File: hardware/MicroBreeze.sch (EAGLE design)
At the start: 43 parts, among them IC1 OPA2251UA, IC3 LM2941TO220-V, IC4 LM2941TO220-V, IC5 ATMEGA328P, J1 COMPUTER-PERIPHERAL-POWERVERT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, Y1 16MHZ

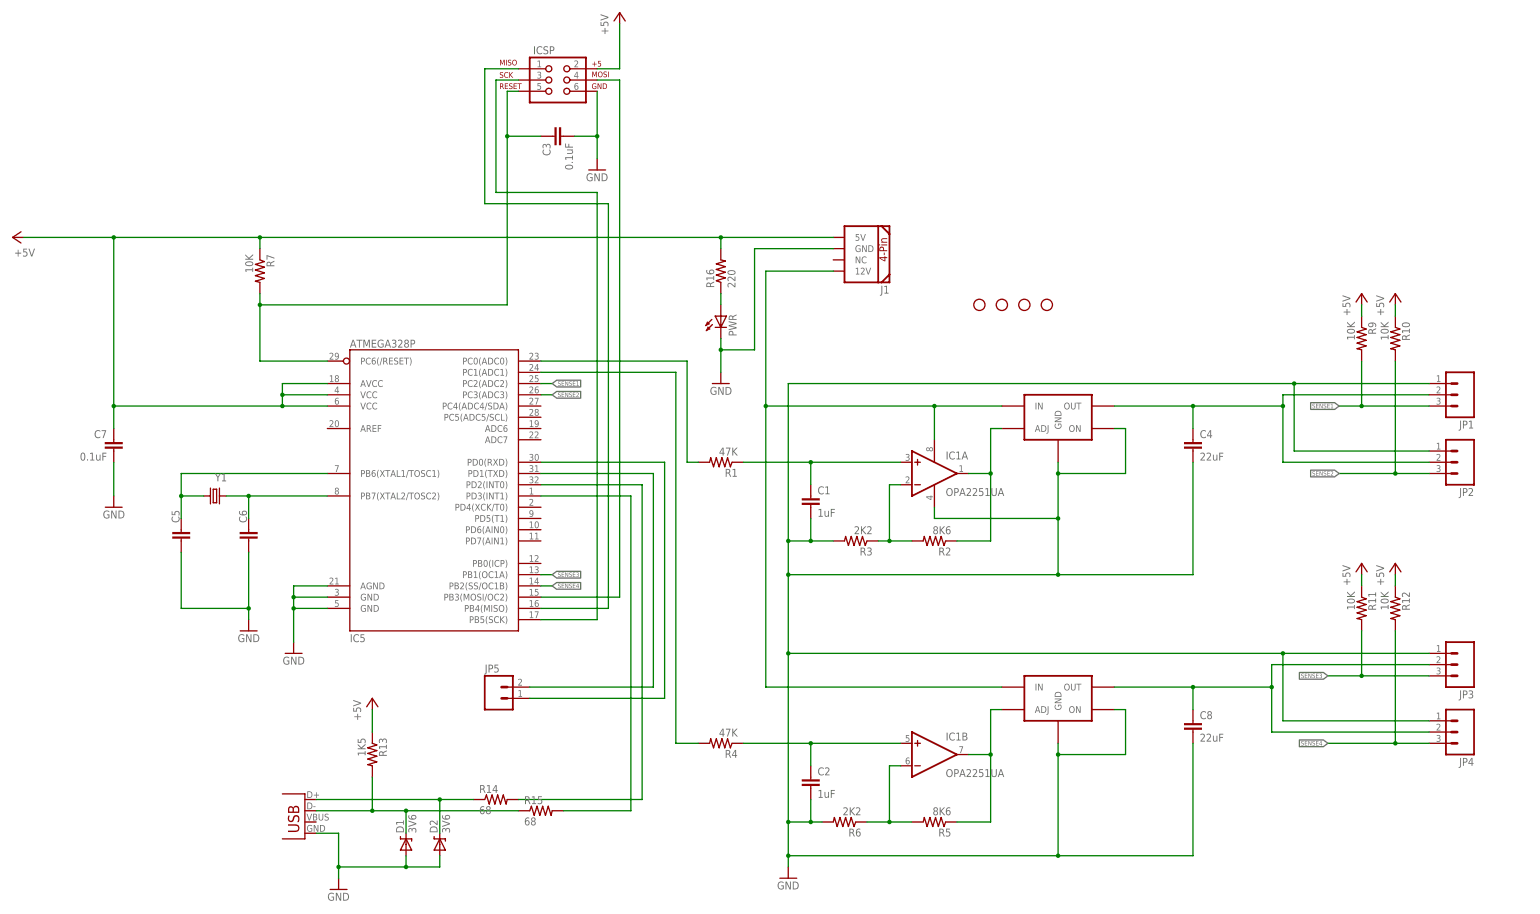
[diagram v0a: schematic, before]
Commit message: Board updates
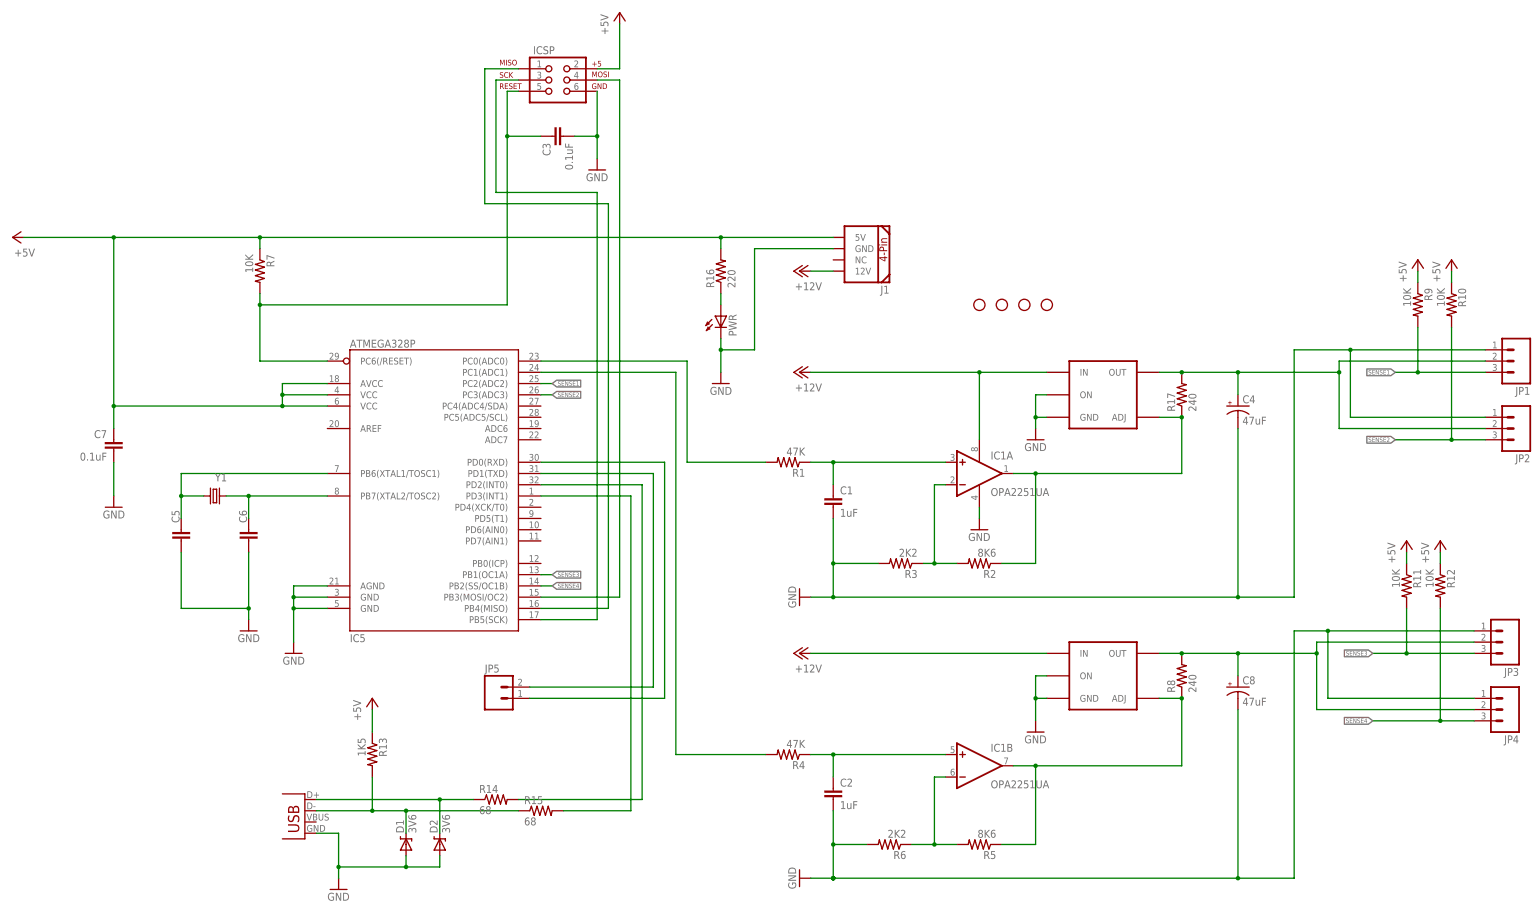
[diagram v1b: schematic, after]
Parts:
- added R17, R8: 240, SparkFun-Resistors:RESISTOR0805-RES
- C4, C8: value 22uF -> 47uF; device SparkFun-Capacitors:22UF-16V-20%-(1210) -> SparkFun-Capacitors:47UF-TANT
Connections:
- removed net N$14: IC1B.OUT, IC4.ADJ, R5.1
- new net N$19: IC1B.OUT, IC4.ADJ, R5.1, R8.1
- net GND: now also C4.-, C8.-; no longer C4.2, C8.2
- net N$13: now also C8.+, R8.2; no longer C8.1
- net N$2: now also R17.1
- net N$8: now also C4.+, R17.2; no longer C4.1
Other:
- moved on the sheet: C1, C2, IC1A, IC1B, JP1, JP2, JP3, JP4, R1, R10, R11, R12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
